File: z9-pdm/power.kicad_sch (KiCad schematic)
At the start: 28 parts, among them U1 B0505XT-1WR3, U22 TLV76733DRVx, U6 LMR14206

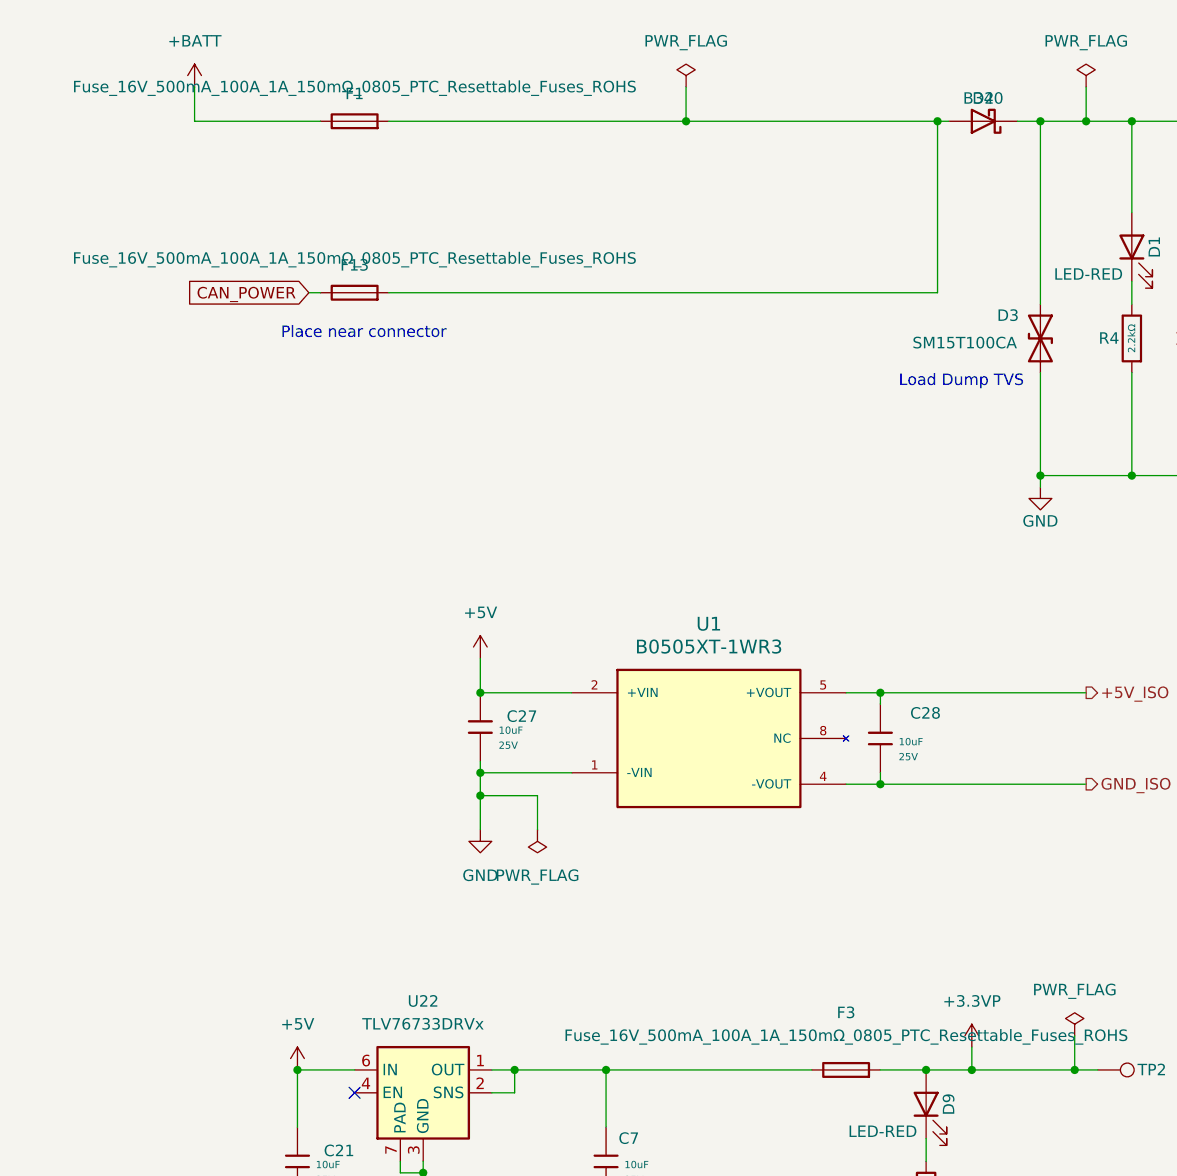
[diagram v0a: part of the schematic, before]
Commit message: x
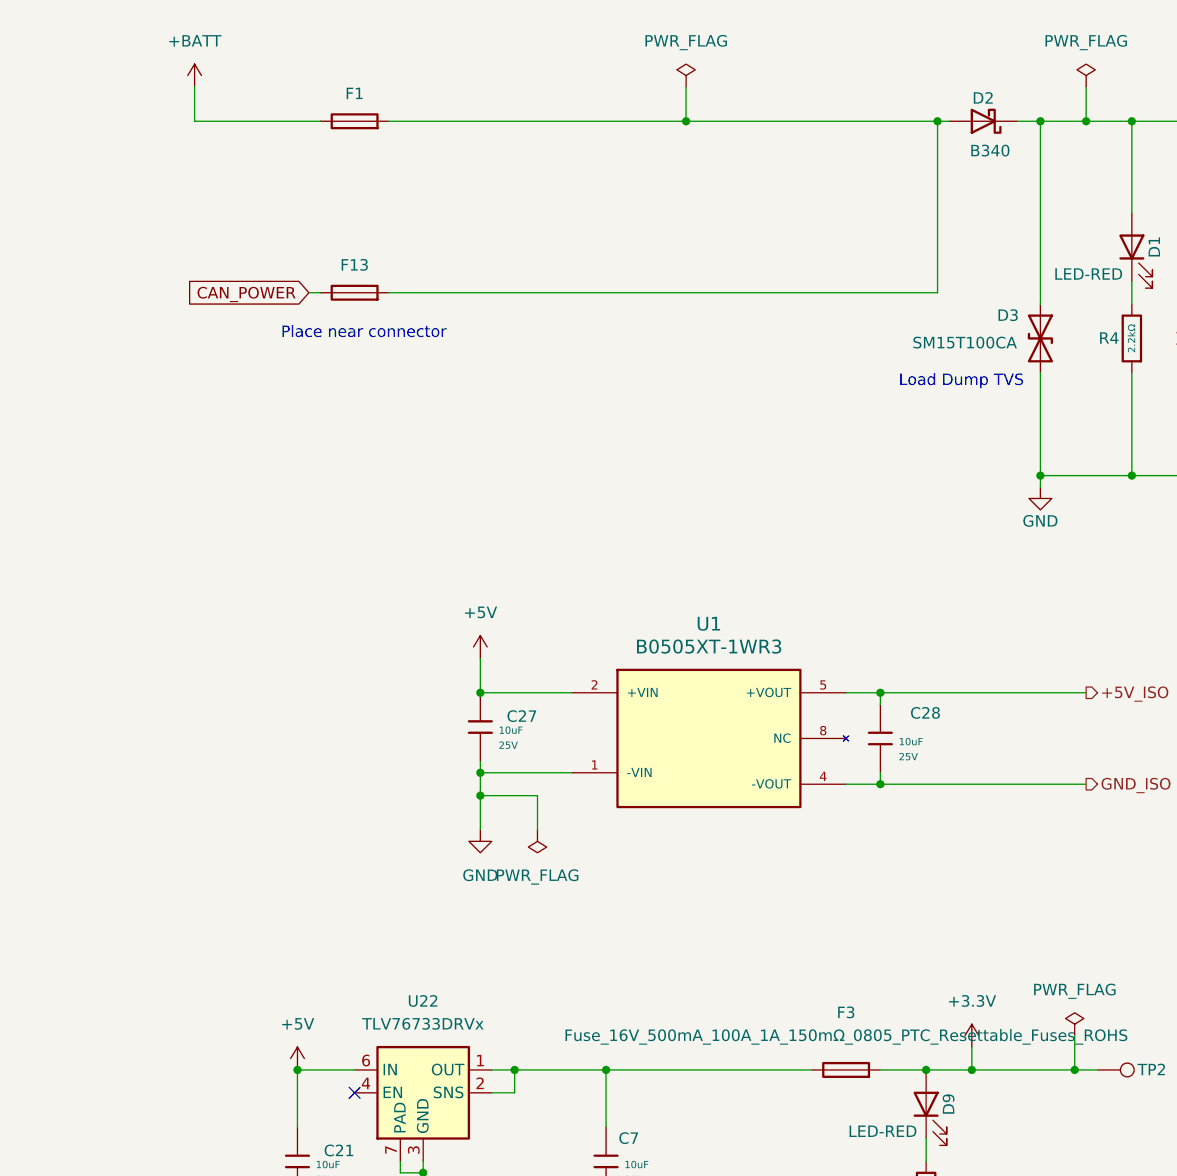
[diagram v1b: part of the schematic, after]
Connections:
- net +3.3VP renamed +3.3V
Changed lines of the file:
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@@
 					(size 1.27 1.27)
 				)
+				(hide yes)
 			)
 		)
@@
 					(size 1.27 1.27)
 				)
+				(hide yes)
 			)
 		)
@@
 		)
 		(property "Value" "B340"
-			(at 105.41 31.75 0)
+			(at 106.172 37.592 0)
 			(effects
 				(font
@@
 			)
 		)
-		(property "Value" "+3.3VP"
+		(property "Value" "+3.3V"
 			(at 104.14 132.08 0)
 			(effects
